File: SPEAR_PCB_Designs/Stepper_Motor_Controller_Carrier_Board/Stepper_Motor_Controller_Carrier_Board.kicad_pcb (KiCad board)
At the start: 2 copper layers, 125.5 x 47 mm, 20 parts, among them J1 Conn_01x02_Pin, J2 Conn_01x02_Pin, J4 JST_S4B-XH-A-1, J5 Conn_01x02_Pin, J6 Conn_01x02_Pin, U1 AP63203WU

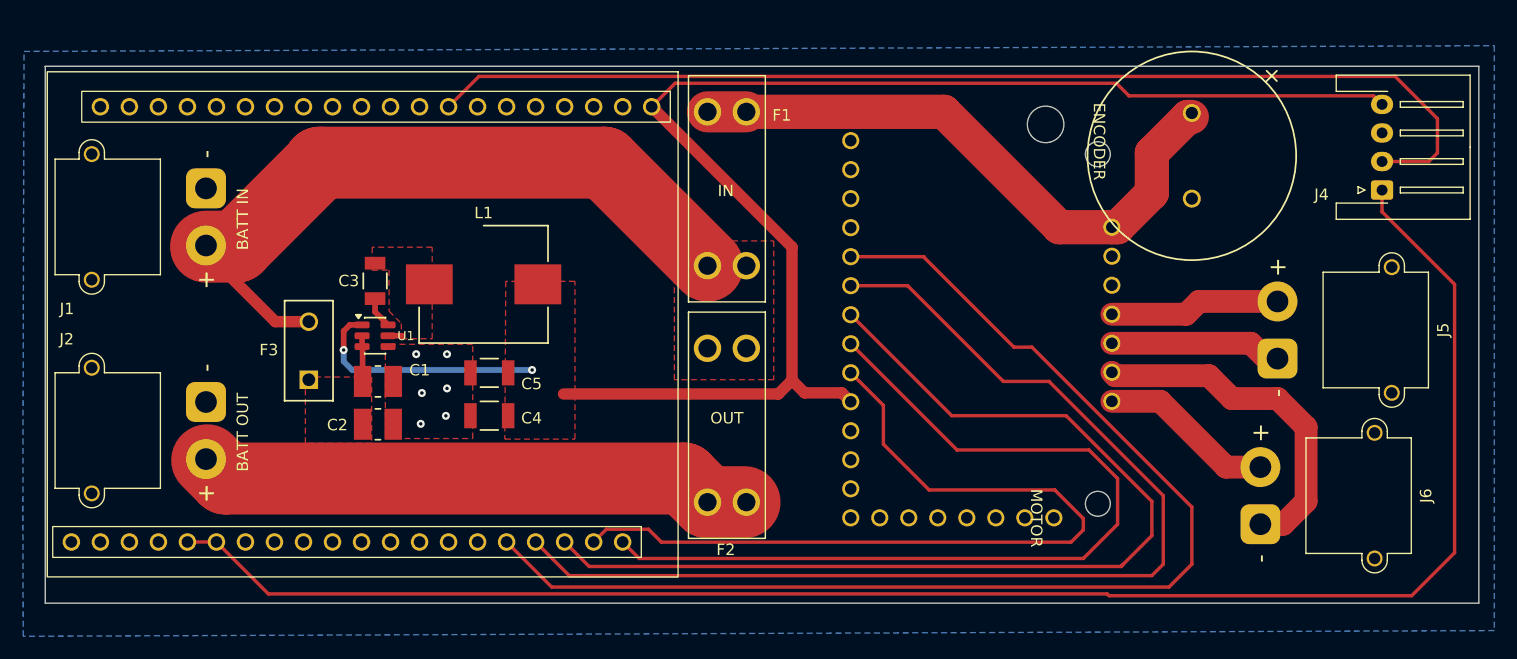
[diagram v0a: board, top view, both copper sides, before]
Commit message: Add files via upload
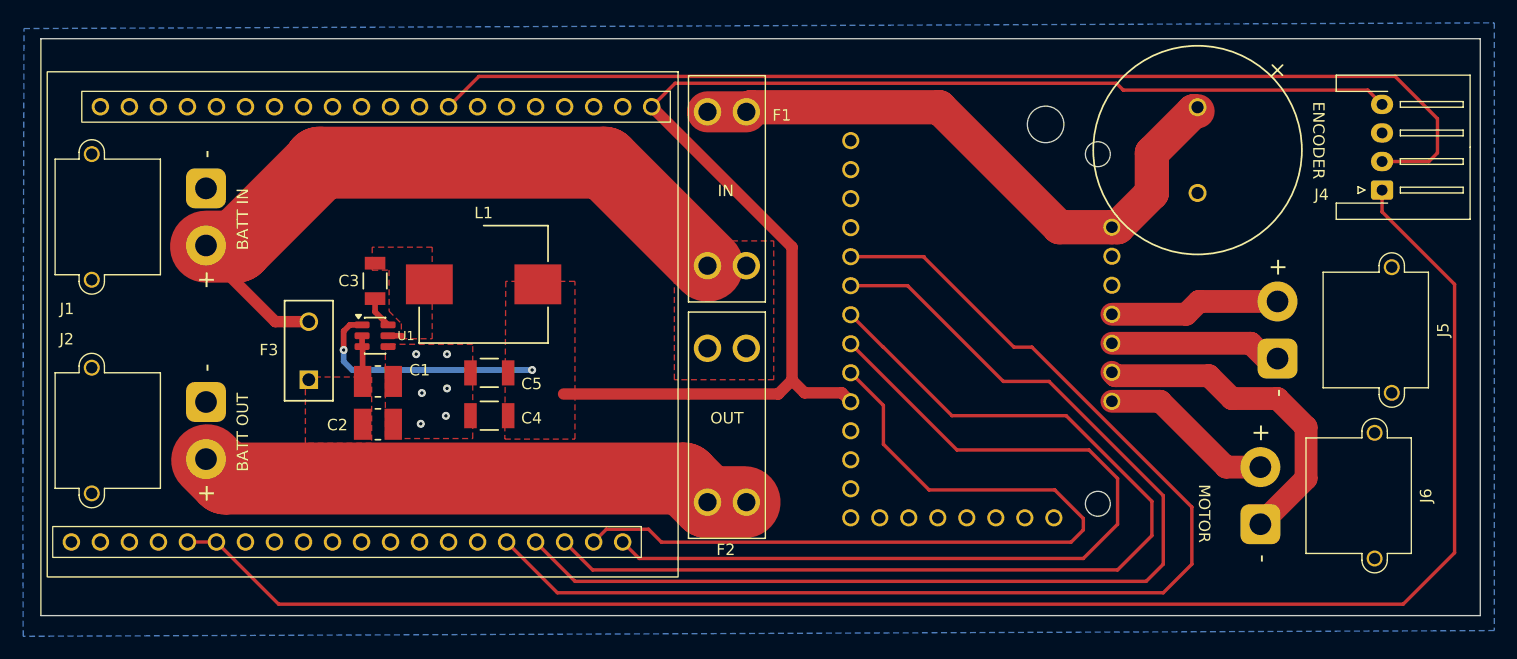
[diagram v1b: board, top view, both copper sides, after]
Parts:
- moved C5 0.71 mm to (188.0, 76.0)
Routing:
- net Net-(J6-Pin_1): track 31.0 -> 29.1 mm
- net /DRIVER_PWR: track 52.6 -> 53.7 mm
- net /ENC_B: track 148.8 -> 149.4 mm
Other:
- board size 125.5 x 47 mm -> 126 x 50.5 mm

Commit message: Add files via upload
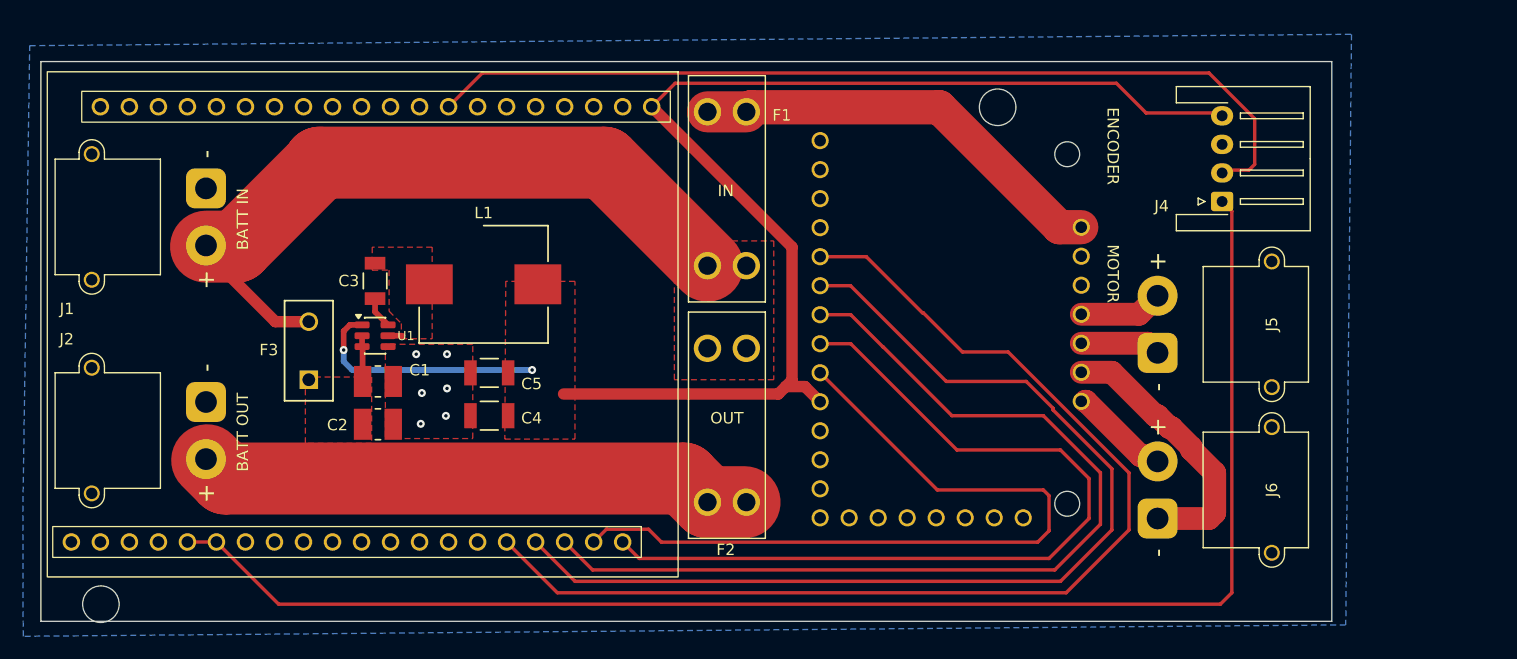
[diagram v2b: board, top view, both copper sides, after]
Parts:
- removed the C5 at (188.0, 76.0)
- added REF**: MountingHole_3.2mm_M3, MountingHole:MountingHole_3.2mm_M3, F.Cu at (92.0, 119.5)
- moved J4 14.0 mm to (190.2, 84.2)
- moved J5 10.5 mm to (184.5, 97.5)
- moved J6 9.01 mm to (184.5, 112.0)
- moved REF** 4.46 mm to (170.5, 76.0)
- moved MDB2 2.68 mm to (153.7, 77.6)
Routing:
- net /ENC_B: track 149.4 -> 129.1 mm
- net /ENC_A: track 97.4 -> 80.6 mm
- net /DRIVER_PWR: track 53.7 -> 37.2 mm
- net +3.3V: track 142.3 -> 126.4 mm
- net /DMODE0: track 106.9 -> 98.5 mm
- net Net-(J5-Pin_2): track 15.0 -> 7.35 mm
- net Net-(J5-Pin_1): track 14.1 -> 7.03 mm
- net /DMODE1: track 98.0 -> 91.4 mm
- net Net-(J6-Pin_2): track 15.4 -> 8.82 mm
- net /DMODE2: track 89.8 -> 84.3 mm
- net Net-(J6-Pin_1): track 29.1 -> 24.1 mm
- net /CLK: track 72.9 -> 68.8 mm
- net /DIR: track 77.4 -> 74.8 mm
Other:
- board size 126 x 50.5 mm -> 113 x 49 mm
- board text added: "Oliver Schneider Ronak Grover Hazem Ammar Henry Diep"
- board text removed: "Oliver Schneider Ronak Grover Henry Diep"
